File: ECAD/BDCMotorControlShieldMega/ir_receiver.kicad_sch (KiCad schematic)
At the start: 6 parts, among them U24 IRM-H6XX, U5 74AHC1G17

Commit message: Progressed ECAD.
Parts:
- C25: footprint Capacitor_SMD:C_0805_2012Metric -> Capacitor_SMD:C_0603_1608Metric; MPN C0805F104K5RACAUTO -> (none)
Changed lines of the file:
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@@
 			)
 		)
-		(property "Footprint" "Capacitor_SMD:C_0805_2012Metric"
+		(property "Footprint" "Capacitor_SMD:C_0603_1608Metric"
 			(at 127.9652 138.43 0)
 			(effects
@@
 			)
 		)
-		(property "Datasheet" "https://www.lcsc.com/datasheet/lcsc_datasheet_2304140030_KEMET-C0805F104K5RACAUTO_C141162.pdf"
+		(property "Datasheet" ""
 			(at 127 134.62 0)
 			(effects
@@
 			)
 		)
-		(property "MPN" "C0805F104K5RACAUTO"
+		(property "MPN" ""
 			(at 127 134.62 0)
 			(effects

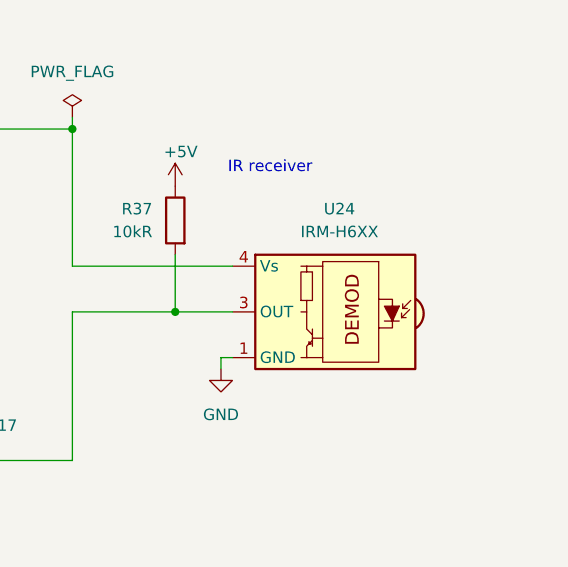
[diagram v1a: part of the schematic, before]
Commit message: Progressed ECAD.
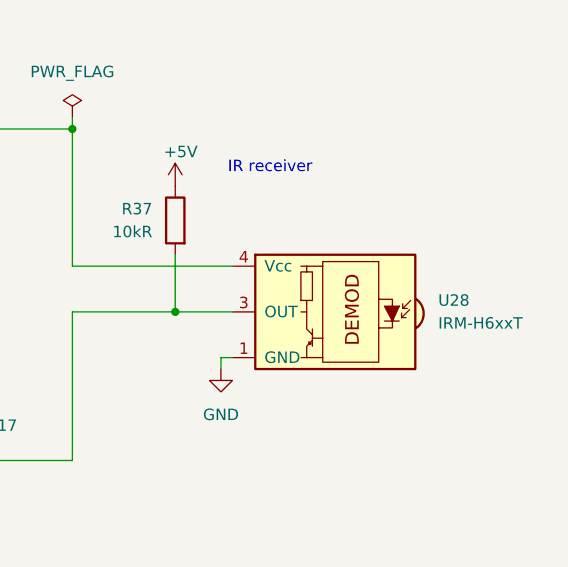
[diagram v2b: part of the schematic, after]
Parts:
- removed U24: IRM-H6XX, OptoDevice_custom:IRM-H6XX, symbol Inteface_Optical_custom:IRM-H6XX
- added U28: IRM-H6xxT, OptoDevice:Everlight_IRM-H6xxT, symbol Interface_Optical:IRM-H6xxT
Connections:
- net GND: now also U28.1 (GND), U28.2 (GND)
- net at R37.2, U5.2: now also U28.3 (OUT)
- net at C57.1, R38.1: now also U28.4 (Vcc)
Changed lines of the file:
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@@
+	)
+	(symbol
+		(lib_id "Interface_Optical:IRM-H6xxT")
+		(at 175.26 88.9 0)
+		(mirror y)
+		(unit 1)
+		(exclude_from_sim no)
+		(in_bom yes)
+		(on_board yes)
+		(dnp no)
+		(fields_autoplaced yes)
+		(property "Reference" "U28"
+			(at 187.96 87.6299 0)
+			(effects
+				(font
+					(size 1.27 1.27)
+				)
+				(justify right)
+			)
+		)
+		(property "Value" "IRM-H6xxT"
+			(at 187.96 90.1699 0)
+			(effects
+				(font
+					(size 1.27 1.27)
+				)
+				(justify right)
+			)
+		)
+		(property "Footprint" "OptoDevice:Everlight_IRM-H6xxT"
+			(at 176.53 98.425 0)
+			(effects
+				(font
+					(size 1.27 1.27)
+				)
+				(hide yes)
+			)
+		)
+		(property "Datasheet" "https://en.everlight.com/wp-content/plugins/ItemRelationship/product_files/pdf/DMO-0000004-IRM-H6XX-TR2_Series_Datasheet_V4.pdf"
+			(at 158.75 81.28 0)
+			(effects
+				(font
+					(size 1.27 1.27)
+				)
+				(hide yes)
+			)
+		)
+		(property "Description" "IR Receiver Modules for remote controls"
+			(at 175.26 88.9 0)
+			(effects
+				(font
+					(size 1.27 1.27)
+				)
+				(hide yes)
+			)
+		)
+		(property "MPN" "IRM-H638J7/TR2(CLW)"
+			(at 175.26 88.9 0)
+			(effects
+				(font
+					(size 1.27 1.27)
+				)
+				(hide yes)
+			)
+		)
+		(pin "3"
+		)
+		(pin "2"
+		)
+		(pin "1"
+		)
+		(pin "4"
+		)
+		(instances
+			(project ""
+				(path "/e63e39d7-6ac0-4ffd-8aa3-1841a4541b55/0406e976-491f-498f-9b04-e9a77bf80632"
+					(reference "U28")
+					(unit 1)
+				)
+			)
+		)
 	)
 	(symbol
@@
 					(unit 1)
 				)
-			)
-		)
-	)
-	(symbol
-		(lib_id "Inteface_Optical_custom:IRM-H6XX")
-		(at 175.26 88.9 0)
-		(mirror y)
-		(unit 1)
-		(exclude_from_sim no)
-		(in_bom yes)
-		(on_board yes)
-		(dnp no)
-		(fields_autoplaced yes)
-		(property "Reference" "U24"
-			(at 176.995 77.47 0)
-			(effects
-				(font
-					(size 1.27 1.27)
-				)
-			)
-		)
-		(property "Value" "IRM-H6XX"
-			(at 176.995 80.01 0)
-			(effects
-				(font
-					(size 1.27 1.27)
-				)
-			)
-		)
-		(property "Footprint" "OptoDevice_custom:IRM-H6XX"
-			(at 176.53 98.425 0)
-			(effects
-				(font
-					(size 1.27 1.27)
-				)
-				(hide yes)
-			)
-		)
-		(property "Datasheet" "https://www.everlight.com/wp-content/plugins/ItemRelationship/product_files/pdf/DMO-0000682_IRM-H6xxJ7-V4.pdf"
-			(at 158.75 81.28 0)
-			(effects
-				(font
-					(size 1.27 1.27)
-				)
-				(hide yes)
-			)
-		)
-		(property "Description" ""
-			(at 175.26 88.9 0)
-			(effects
-				(font
-					(size 1.27 1.27)
-				)
-			)
-		)
-		(property "MPN" "IRM-H638J7/TR2(CLW)"
-			(at 175.26 88.9 0)
-			(effects
-				(font
-					(size 1.27 1.27)
-				)
-				(hide yes)
-			)
-		)
-		(property "Status" "OK"
-			(at 175.26 88.9 0)
-			(effects
-				(font
-					(size 1.27 1.27)
-				)
-				(hide yes)
-			)
-		)
-		(pin "1"
-		)
-		(pin "2"
-		)
-		(pin "3"
-		)
-		(pin "4"
-		)
-		(instances
-			(project "BDCMotorControlShieldMega"
-				(path "/e63e39d7-6ac0-4ffd-8aa3-1841a4541b55/0406e976-491f-498f-9b04-e9a77bf80632"
-					(reference "U24")
-					(unit 1)
-				)
